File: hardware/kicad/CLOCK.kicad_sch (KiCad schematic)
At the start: 14 parts, among them J2 Ext Res, J3 Ext CLK, SW2 Reset, U5 8284, Y1 14.31818 MHz

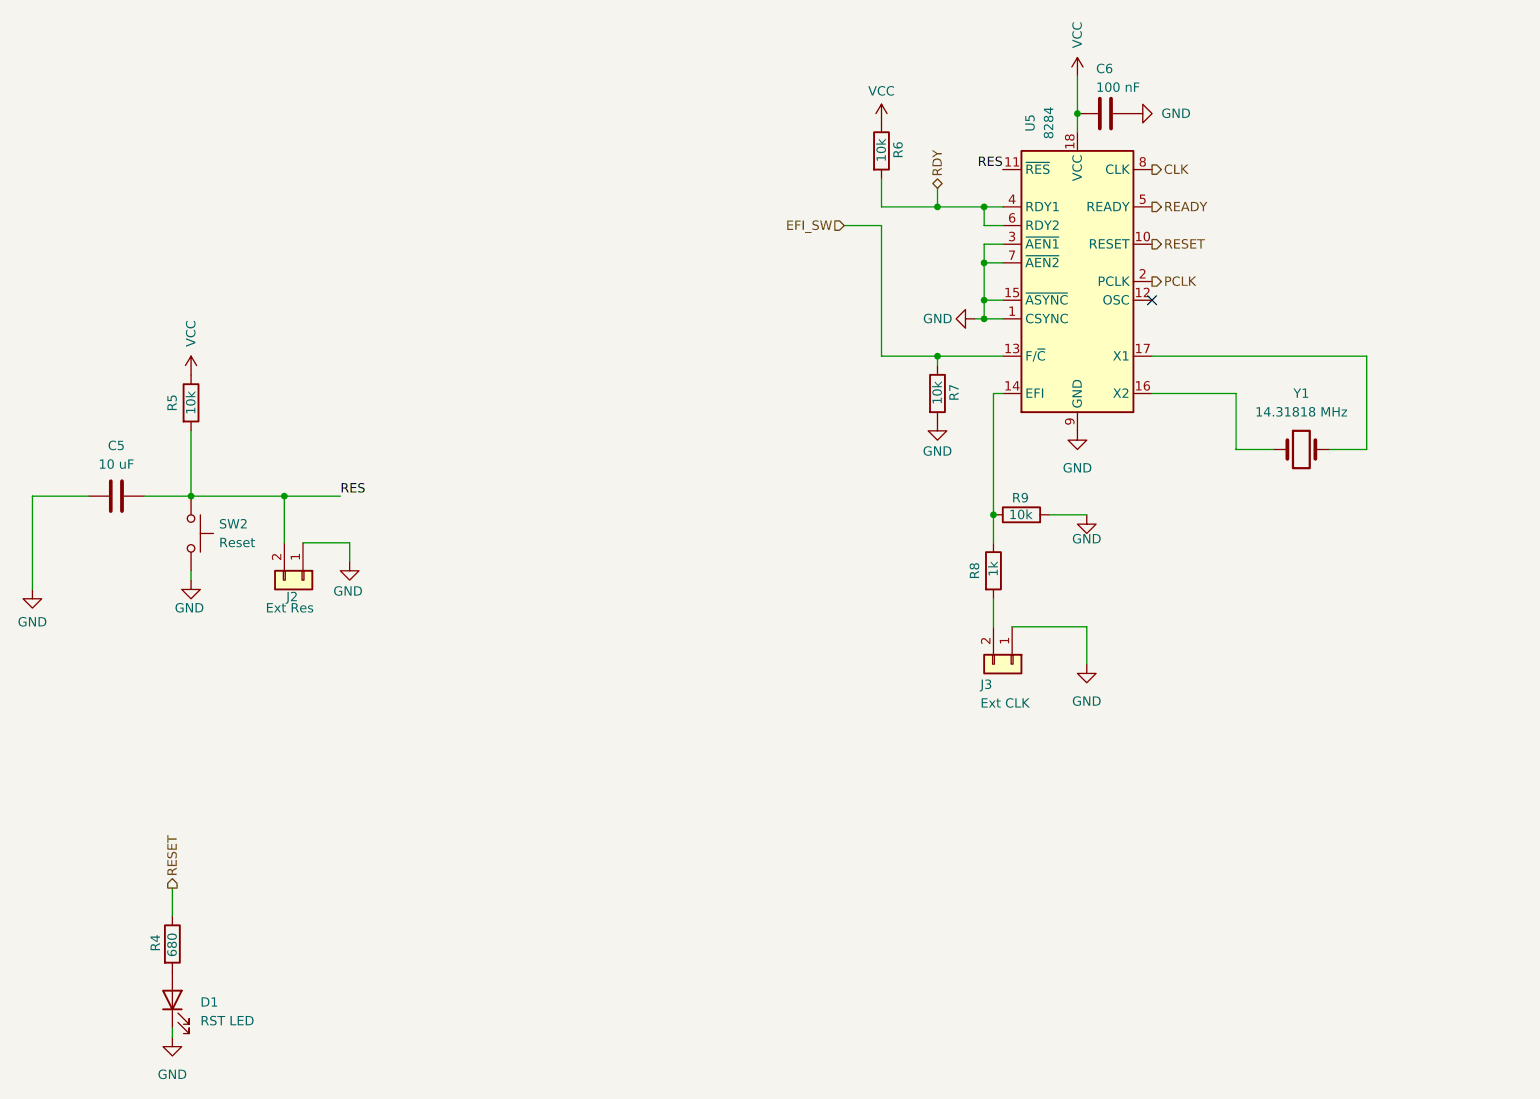
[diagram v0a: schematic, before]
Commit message: Update schema
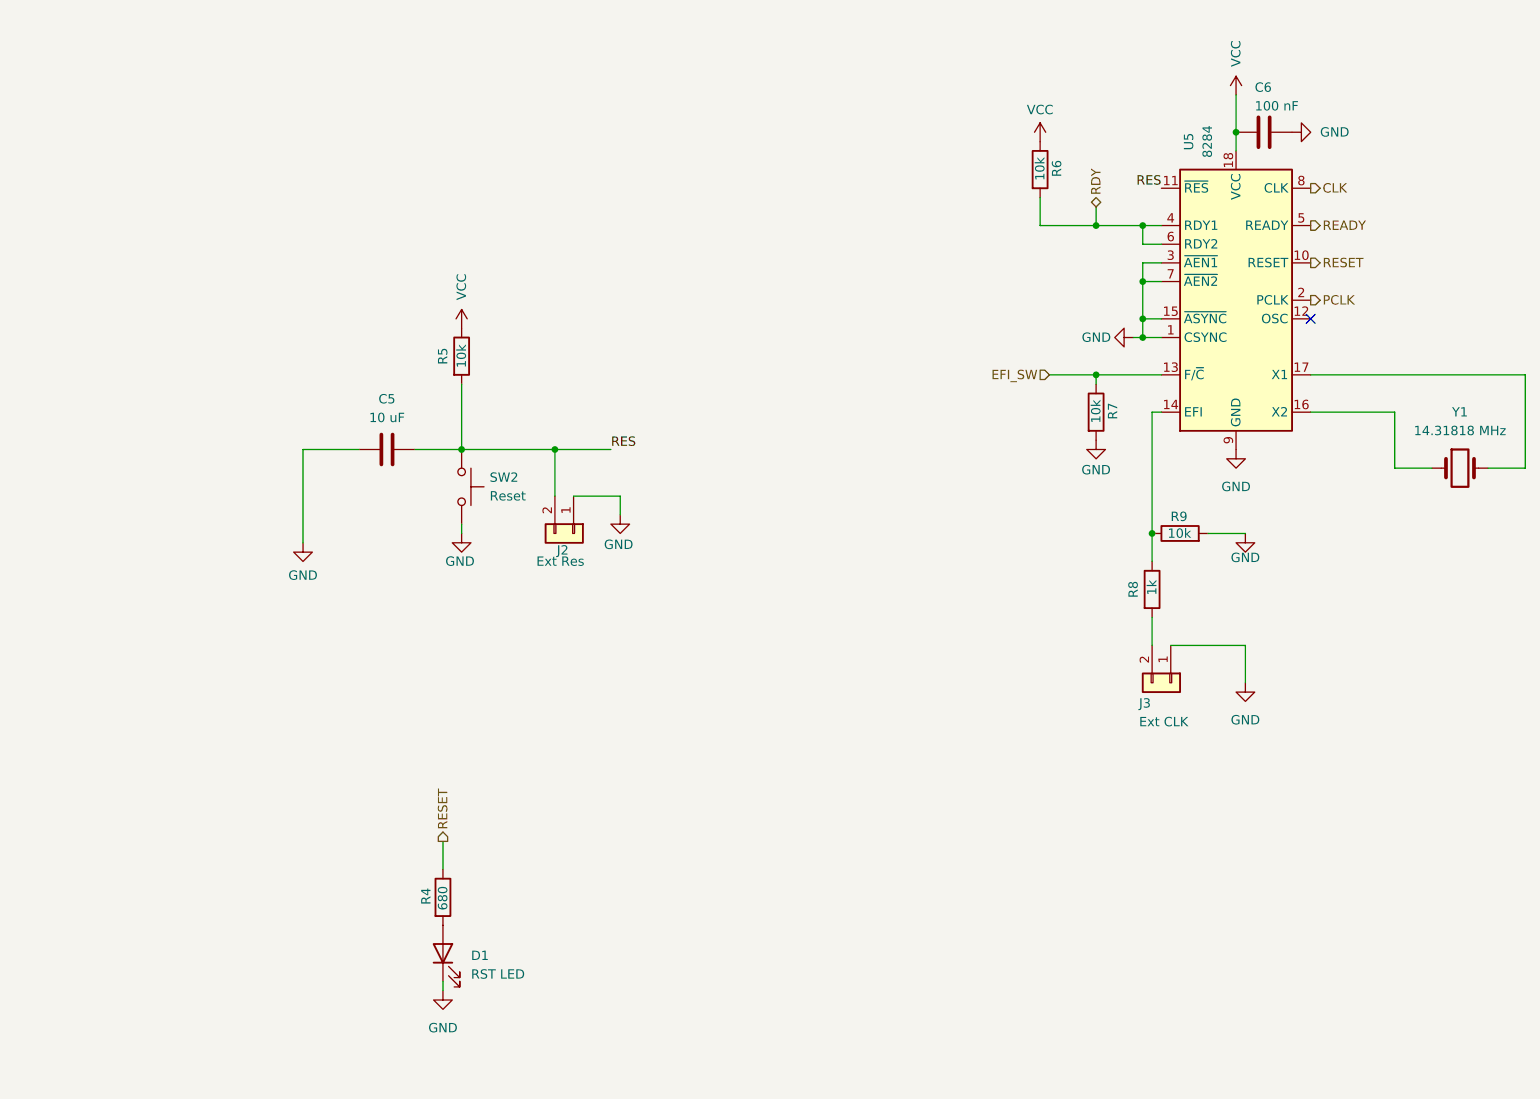
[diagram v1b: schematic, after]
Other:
- moved on the sheet: C5, C6, D1, J2, J3, R4, R5, R6, R7, R8, R9, SW2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
